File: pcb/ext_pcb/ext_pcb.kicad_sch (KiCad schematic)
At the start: 6 parts, among them J1 SFW15R-2STE1LF, J2 Conn_01x04_Pin, J3 Conn_01x04_Pin, J4 SJ2-3574A-SMT-TR, J5 Conn_02x07_Counter_Clockwise

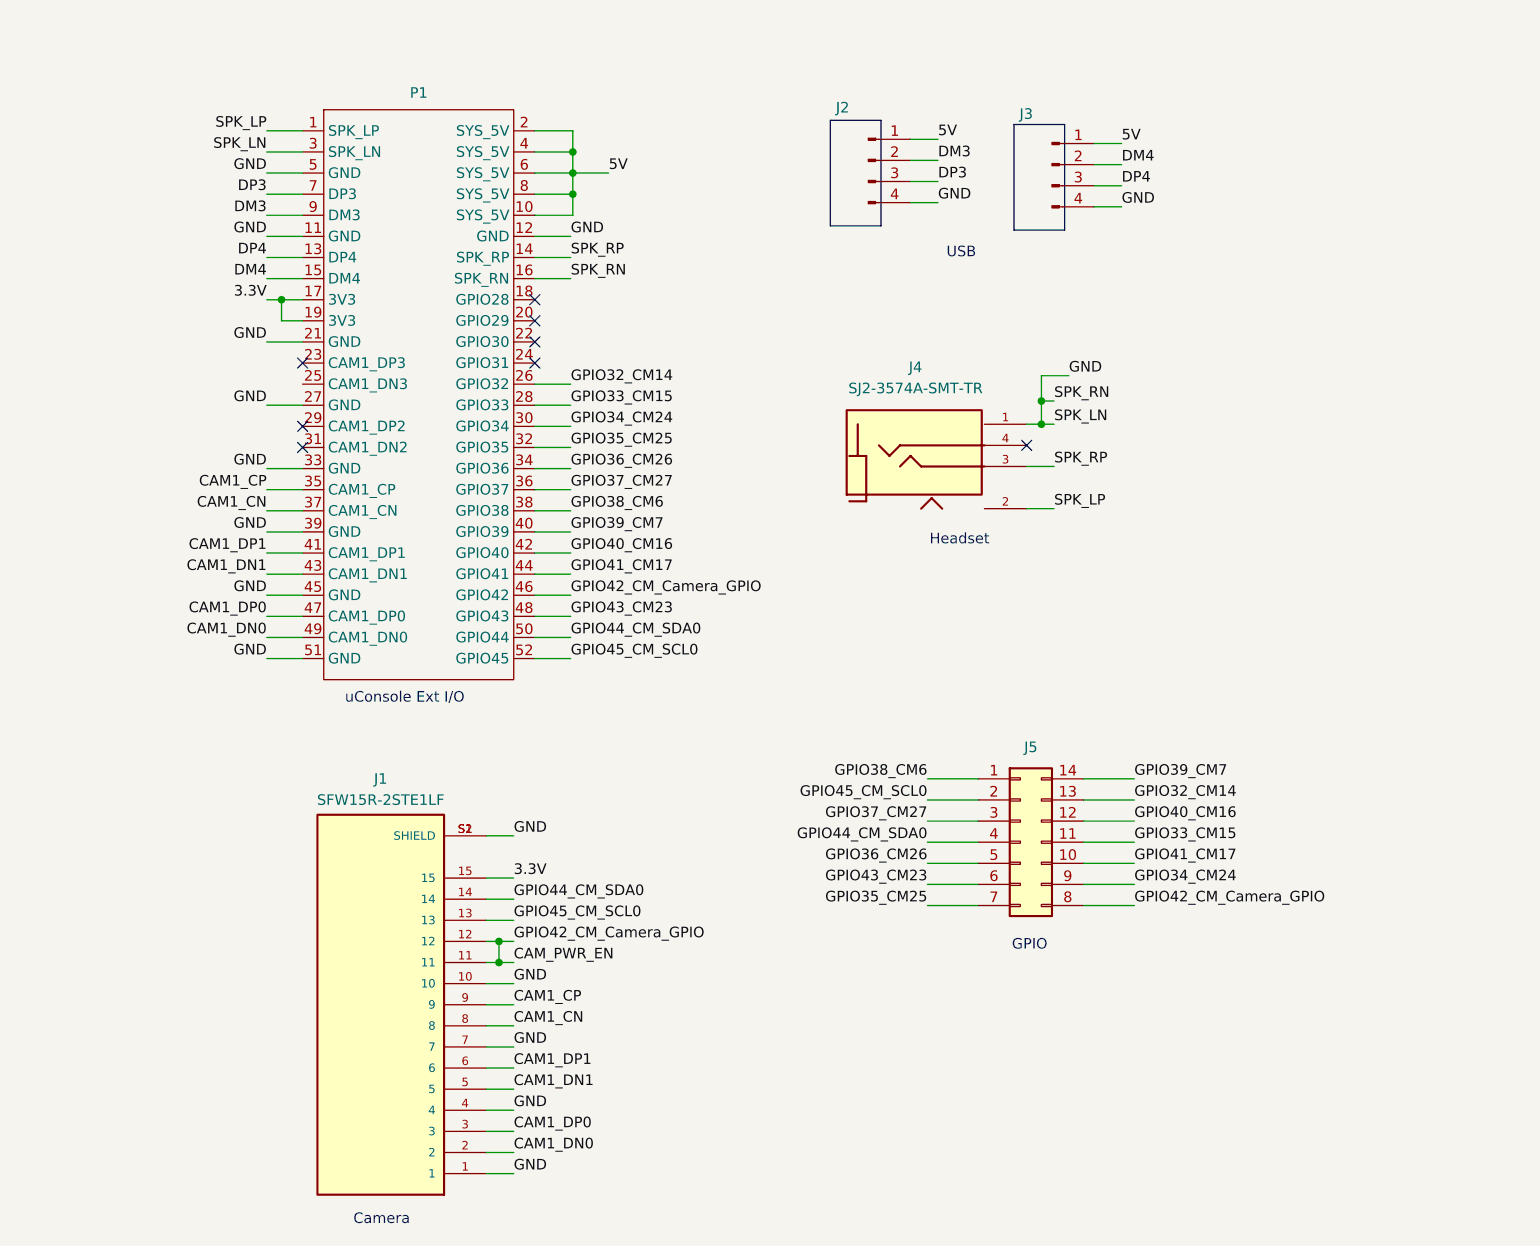
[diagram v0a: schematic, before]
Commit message: REV: A
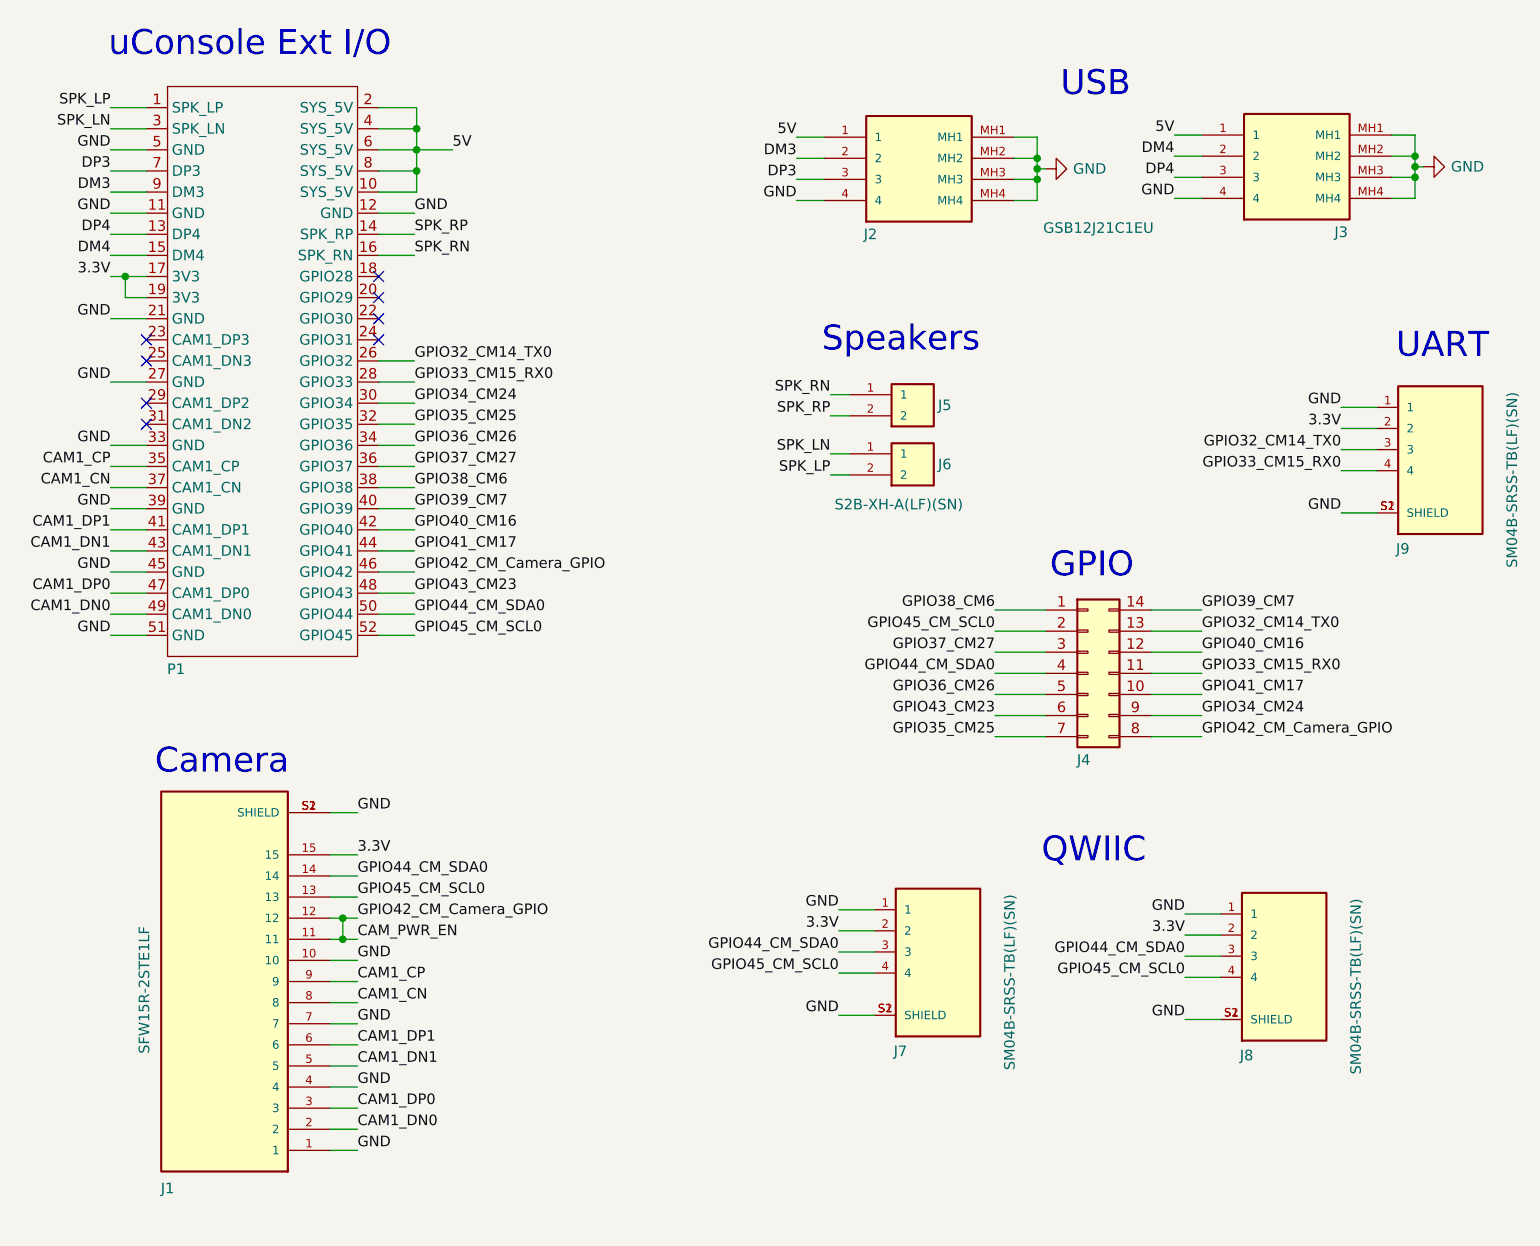
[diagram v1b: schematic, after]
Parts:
- removed J2, J3: Conn_01x04_Pin, 1_project:USB_TYPE_A, symbol Connector:Conn_01x04_Pin
- removed J4: SJ2-3574A-SMT-TR, 1_project:CUI_SJ2-3574A-SMT-TR, symbol 1_project:SJ2-3574A-SMT-TR
- added J2, J3: GSB12J21C1EU, 1_project:GSB12J21C1EU, symbol 1_project:GSB12J21C1EU
- added J5, J6: S2B-XH-A(LF)(SN), 1_project:JST_S2B-XH-A(LF)(SN), symbol 1_project:S2B-XH-A(LF)(SN)
- added J7, J8, J9: SM04B-SRSS-TB(LF)(SN), 1_project:JST_SM04B-SRSS-TB(LF)(SN), symbol 1_project:SM04B-SRSS-TB(LF)(SN)
- renumbered J5 to J4
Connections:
- net 3.3V: now also J7.2, J8.2, J9.2
- net 5V: now also J2.1, J3.1
- net DM3: now also J2.2
- net DM4: now also J3.2
- net DP3: now also J2.3
- net DP4: now also J3.3
- net GND: now also J2.4, J2.MH1, J2.MH2, J2.MH3, J2.MH4, J3.4, J3.MH1, J3.MH2, J3.MH3, J3.MH4, J7.1, J7.S1 (SHIELD), J7.S2 (SHIELD), J8.1, J8.S1 (SHIELD), J8.S2 (SHIELD), J9.1, J9.S1 (SHIELD), J9.S2 (SHIELD); no longer P1.16 (SPK_RN), P1.3 (SPK_LN)
- net GPIO44_CM_SDA0: now also J7.3, J8.3
- net GPIO45_CM_SCL0: now also J7.4, J8.4
- net SPK_LP: now also J6.2
- net SPK_RP: now also J5.2
- net GPIO32_CM14 renamed GPIO32_CM14_TX0
- net GPIO32_CM14_TX0: now also J9.3
- net GPIO33_CM15 renamed GPIO33_CM15_RX0
- net GPIO33_CM15_RX0: now also J9.4
- new net SPK_LN: J6.1, P1.3 (SPK_LN)
- new net SPK_RN: J5.1, P1.16 (SPK_RN)
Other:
- note added: "QWIIC"
- note added: "Speakers"
- note added: "UART"
- note removed: "Headset"
- moved on the sheet: J1, J4, P1
